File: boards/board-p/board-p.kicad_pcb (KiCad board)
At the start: 0 parts

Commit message: update
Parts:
- added C1: 10uF/50V, zudo-led-lamp:C1206, F.Cu at (128.5, 79.5)
- added C2: 100nF/50V, zudo-led-lamp:C0603, F.Cu at (142.0, 87.9)
- added C30: 1uF/50V, zudo-led-lamp:C0603, F.Cu at (142.0, 89.9)
- added C34: 1uF/50V, zudo-led-lamp:C0603, F.Cu at (142.0, 95.2)
- added C35: 100nF/50V, zudo-led-lamp:C0603, F.Cu at (146.8, 81.3)
- added D5: SMAJ20A, zudo-led-lamp:SMA_L4.2-W2.6-LS5.3-RD, F.Cu at (147.6, 77.0)
- added D6: PESD24VS1UB, zudo-led-lamp:SOD-523_L1.2-W0.8-LS1.6-RD, F.Cu at (137.0, 83.6)
- added D7: PESD24VS1UB, zudo-led-lamp:SOD-523_L1.2-W0.8-LS1.6-RD, F.Cu at (129.5, 83.6)
- added J1: TYPE-C-31-M-17, zudo-led-lamp:USB-C-SMD_10P-P1.00-L6.8-W8.9, F.Cu at (138.2, 72.4)
- added J2: PogoPad_1x4_NVM_I2C, zudo-led-lamp:PogoPad_1x04_P2.54mm, F.Cu at (127.8, 96.9)
- added J3: PogoPad_1x8_Debug, zudo-led-lamp:PogoPad_1x08_P2.54mm, F.Cu at (150.1, 94.2)
- added JOUT1: 2.54mm 1x6 male, zudo-led-lamp:HDR-TH_6P-P2.54-V-M, F.Cu at (137.7, 104.6)
- added Q1: AO3401A, zudo-led-lamp:SOT-23_L2.9-W1.3-P1.90-LS2.4-BR, F.Cu at (143.3, 80.5)
- added R11: 100k, zudo-led-lamp:R0603, F.Cu at (146.8, 83.1)
- added R12: 150k, zudo-led-lamp:R0603, F.Cu at (148.1, 79.5)
- added R13: 470R, zudo-led-lamp:R0603, F.Cu at (130.3, 90.2)
- added R14: 470R, zudo-led-lamp:R0603, F.Cu at (140.5, 84.1)
- added R15: 4.7k, zudo-led-lamp:R0603, F.Cu at (142.0, 93.5)
- added R16: 4.7k, zudo-led-lamp:R0603, F.Cu at (142.0, 91.7)
- added R17: 5.1k, zudo-led-lamp:R0603, F.Cu at (135.4, 83.6)
- added R18: 5.1k, zudo-led-lamp:R0603, F.Cu at (131.8, 83.6)
- added R19: 0R, zudo-led-lamp:R0603, F.Cu at (138.7, 84.1)
- added R20: 0R, zudo-led-lamp:R0603, F.Cu at (133.5, 83.6)
- added R21: 10k, zudo-led-lamp:R0805, F.Cu at (129.0, 87.4)
- added REF**: MountingHole_3.2mm_M3, MountingHole:MountingHole_3.2mm_M3, F.Cu at (129.5, 71.9)
- added REF**: MountingHole_3.2mm_M3, MountingHole:MountingHole_3.2mm_M3, F.Cu at (137.4, 99.3)
- added REF**: MountingHole_3.2mm_M3, MountingHole:MountingHole_3.2mm_M3, F.Cu at (147.3, 71.9)
- added U1: STUSB4500QTR, zudo-led-lamp:QFN-24_L4.0-W4.0-P0.50-BL-EP2.8, F.Cu at (136.4, 90.2)
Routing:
- net GND: track 0.00 -> 67.5 mm, vias 0 -> 37
- net VBUS_IN: track 0.00 -> 66.4 mm, vias 0 -> 2
- net VBUS_OUT: track 0.00 -> 53.7 mm, vias 0 -> 3
- net VBEN: track 0.00 -> 42.8 mm, vias 0 -> 2
- net SCL: track 0.00 -> 39.1 mm, vias 0 -> 4
- net ATT: track 0.00 -> 34.3 mm, vias 0 -> 2
- net SDA: track 0.00 -> 32.7 mm, vias 0 -> 3
- net PDOK: track 0.00 -> 25.4 mm, vias 0 -> 2
- net VBUS_VS_DISCH: track 0.00 -> 23.6 mm, vias 0 -> 4
- net CC2DB: track 0.00 -> 21.0 mm, vias 0 -> 3
- net CC2: track 0.00 -> 20.8 mm
- net CC1: track 0.00 -> 16.7 mm
- net CC1DB: track 0.00 -> 16.3 mm, vias 0 -> 2
- net VREG_2V7: track 0.00 -> 15.9 mm
- net Q1_G: track 0.00 -> 14.5 mm
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- added copper zone on B.Cu, net GND
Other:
- board outline added: 26.4 x 39.6 mm
- copper layers 0 -> 2

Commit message: update
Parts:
- moved J2 142.7 mm to (1.80, 29.8)
- moved REF** 142.7 mm to (4.00, 4.00)
- moved D5 142.1 mm to (22.2, 10.1)
- moved J1 141.7 mm to (13.5, 5.00)
- moved J3 141.7 mm to (25.2, 27.4)
- moved REF** 141.6 mm to (23.0, 4.00)
- moved C35 141.5 mm to (22.1, 14.4)
- moved D7 141.5 mm to (4.87, 16.7)
- moved R11 141.5 mm to (22.1, 16.2)
- moved R13 141.5 mm to (5.63, 23.3)
- moved R14 141.5 mm to (15.8, 17.2)
- moved R18 141.5 mm to (7.13, 16.7)
- moved R21 141.5 mm to (4.36, 20.5)
- moved C1 141.5 mm to (3.85, 12.6)
- moved C2 141.5 mm to (17.4, 21.0)
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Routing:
- net GND: track 67.5 -> 60.9 mm, vias 37 -> 21
- net RESET: track 13.7 -> 15.1 mm
- net SDA: track 32.7 -> 34.1 mm
- net SCL: track 39.1 -> 39.9 mm
- net VBUS_IN: track 66.4 -> 67.2 mm
- net CC1: track 16.7 -> 17.3 mm
- net CC2: track 20.8 -> 21.3 mm
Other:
- board size 26.4 x 39.6 mm -> 27 x 40 mm

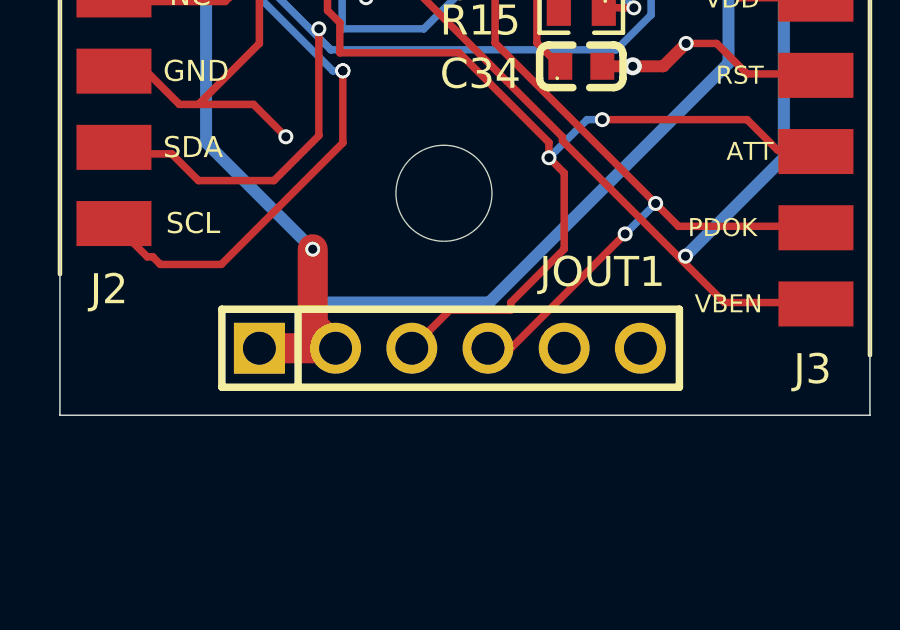
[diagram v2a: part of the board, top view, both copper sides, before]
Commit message: forgot to commit
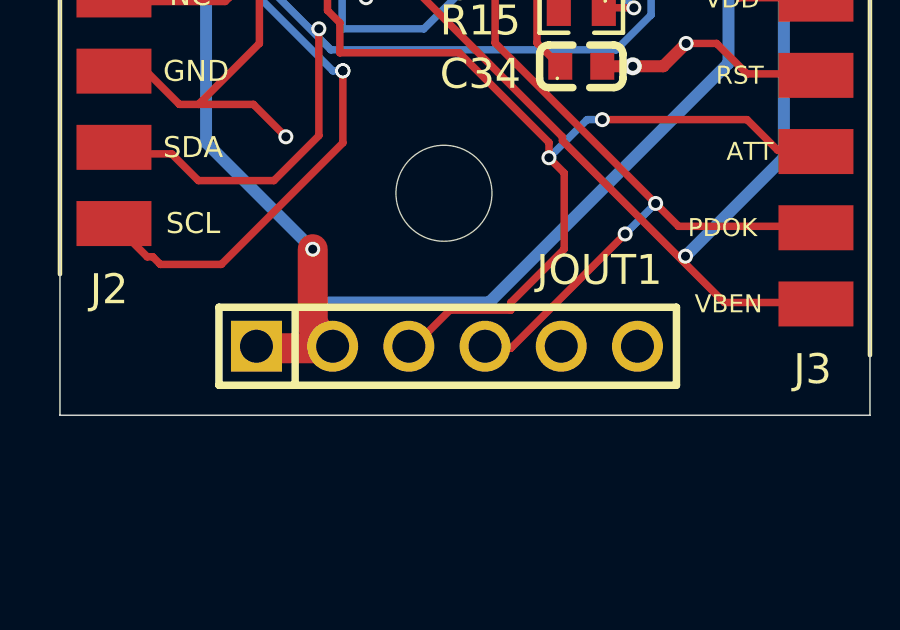
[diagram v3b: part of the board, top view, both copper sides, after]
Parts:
- moved JOUT1 0.12 mm to (12.9, 37.7)
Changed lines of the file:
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@@
 		(capping no)
 		(filling no)
-		(zone_defaults)
 		(pcbplotparams
 			(layerselection 0x00000000_00000000_55555555_5755f5ff)
@@
 	(footprint "zudo-led-lamp:HDR-TH_6P-P2.54-V-M"
 		(layer "F.Cu")
-		(at 12.998 37.766)
+		(at 12.9 37.7)
 		(property "Reference" "JOUT1"
 			(at 5.08 -2.54 0)
